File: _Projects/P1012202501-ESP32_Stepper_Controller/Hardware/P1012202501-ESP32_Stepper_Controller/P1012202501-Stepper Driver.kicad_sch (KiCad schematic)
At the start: 17 parts, among them CN6 KHS4B-PH-SM4-TB(LF)(SN), CN7 KPTBP04R1-500-04BE, IC6 UDRV8825PWPR

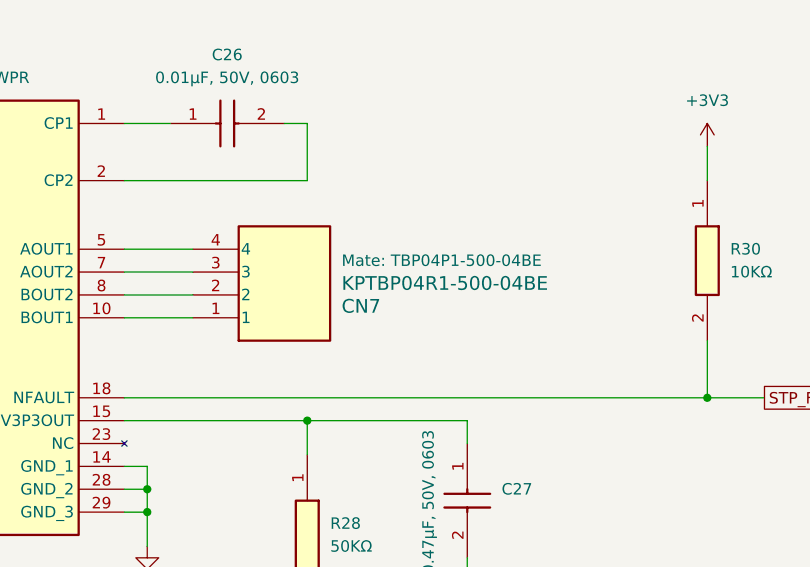
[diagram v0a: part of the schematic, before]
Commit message: Added new content and changes from stream.
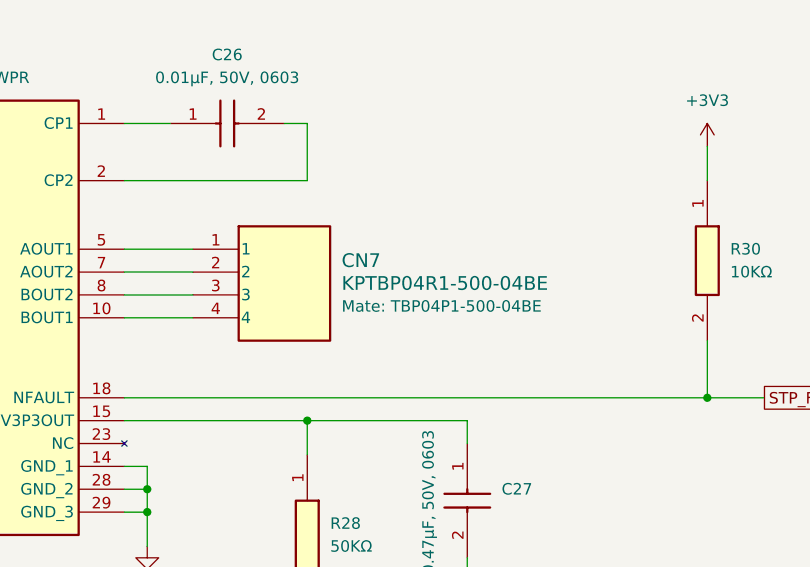
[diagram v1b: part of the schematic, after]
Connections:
- net at CN7.1: now also IC6.5 (AOUT1); no longer IC6.10 (BOUT1)
- net at CN7.2: now also IC6.7 (AOUT2); no longer IC6.8 (BOUT2)
- net at CN7.3: now also IC6.8 (BOUT2); no longer IC6.7 (AOUT2)
- net at CN7.4: now also IC6.10 (BOUT1); no longer IC6.5 (AOUT1)

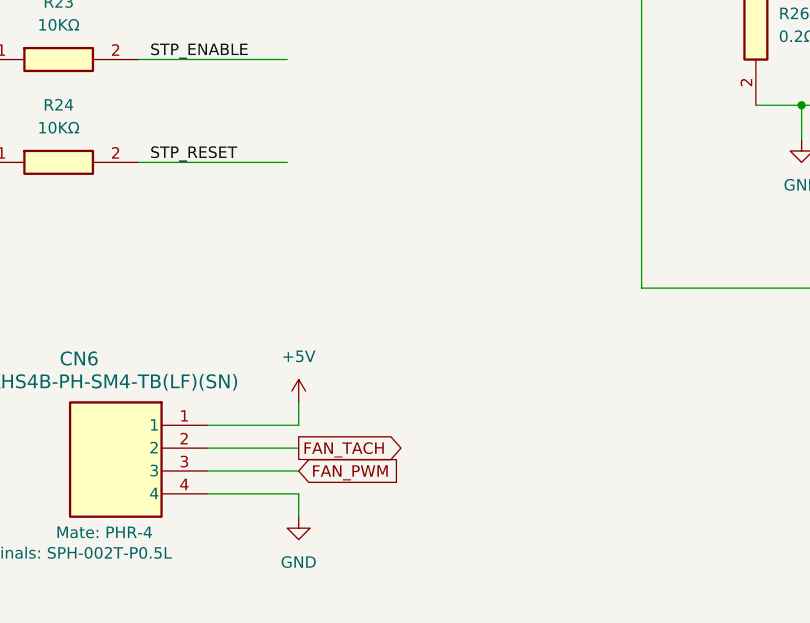
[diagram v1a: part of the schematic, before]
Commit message: Added items from latest stream.
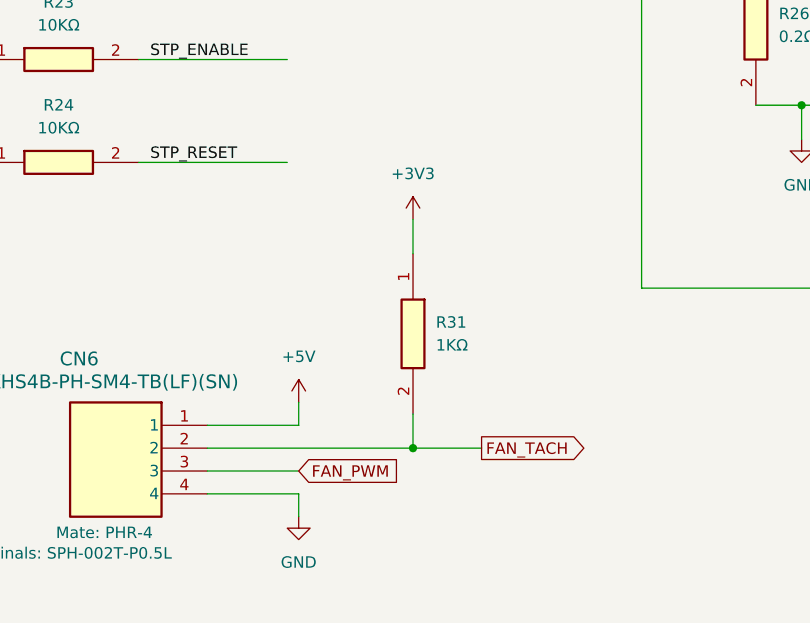
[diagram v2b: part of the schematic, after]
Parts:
- added R31: RC06031K0075AAA, COMPONENTS:RES-0603, symbol COMPONENTS:RC06031K0075AAA
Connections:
- net +3V3: now also R31.1
- net FAN_TACH: now also R31.2
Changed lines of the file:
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@@
 	)
 	(junction
+		(at 80.01 171.45)
+		(diameter 0)
+		(color 0 0 0 0)
+	)
+	(junction
 		(at 72.39 69.85)
 		(diameter 0)
@@
 	(wire
 		(pts
+			(xy 80.01 146.05) (xy 80.01 149.86)
+		)
+		(stroke
+			(width 0)
+			(type default)
+		)
+	)
+	(wire
+		(pts
 			(xy 170.18 113.03) (xy 172.72 113.03)
 		)
@@
 	(wire
 		(pts
+			(xy 80.01 171.45) (xy 87.63 171.45)
+		)
+		(stroke
+			(width 0)
+			(type default)
+		)
+	)
+	(wire
+		(pts
 			(xy 105.41 106.68) (xy 105.41 153.67)
 		)
@@
 	(wire
 		(pts
-			(xy 57.15 171.45) (xy 67.31 171.45)
+			(xy 57.15 171.45) (xy 80.01 171.45)
 		)
 		(stroke
@@
 	(wire
 		(pts
+			(xy 80.01 167.64) (xy 80.01 171.45)
+		)
+		(stroke
+			(width 0)
+			(type default)
+		)
+	)
+	(wire
+		(pts
 			(xy 234.95 72.39) (xy 234.95 76.2)
 		)
@@
 	(global_label "FAN_TACH"
 		(shape output)
-		(at 67.31 171.45 0)
+		(at 87.63 171.45 0)
 		(fields_autoplaced yes)
 		(effects
@@
 		)
 		(property "Intersheetrefs" "${INTERSHEET_REFS}"
-			(at 79.4272 171.45 0)
+			(at 99.7472 171.45 0)
 			(effects
 				(font
@@
 	)
 	(symbol
+		(lib_id "COMPONENTS:RC06031K0075AAA")
+		(at 80.01 149.86 270)
+		(unit 1)
+		(exclude_from_sim no)
+		(in_bom yes)
+		(on_board yes)
+		(dnp no)
+		(fields_autoplaced yes)
+		(property "Reference" "R31"
+			(at 82.55 157.4799 90)
+			(effects
+				(font
+					(size 1.27 1.27)
+				)
+				(justify left)
+			)
+		)
+		(property "Value" "RC06031K0075AAA"
+			(at 73.914 151.384 0)
+			(effects
+				(font
+					(size 1.27 1.27)
+				)
+				(justify left top)
+				(hide yes)
+			)
+		)
+		(property "Footprint" "COMPONENTS:RES-0603"
+			(at -16.18 163.83 0)
+			(effects
+				(font
+					(size 1.27 1.27)
+				)
+				(justify left top)
+				(hide yes)
+			)
+		)
+		(property "Datasheet" ""
+			(at -116.18 163.83 0)
+			(effects
+				(font
+					(size 1.27 1.27)
+				)
+				(justify left top)
+				(hide yes)
+			)
+		)
+		(property "Description" "Resistor, Chip, 0603, 1KΩ, 75V, 5%, -55°C to 155°C, RoHS, AEC-Q200"
+			(at 70.866 153.924 0)
+			(effects
+				(font
+					(size 1.27 1.27)
+				)
+				(hide yes)
+			)
+		)
+		(property "Manufacturer 1" "Yageo"
+			(at 64.516 147.32 0)
+			(effects
+				(font
+					(size 1.27 1.27)
+				)
+				(hide yes)
+			)
+		)
+		(property "Manufacturer 1 P/N" "SR0603JR-071KL"
+			(at 66.802 156.972 0)
+			(effects
+				(font
+					(size 1.27 1.27)
+				)
+				(hide yes)
+			)
+		)
+		(property "Vendor 1a" "Mouser"
+			(at 82.296 130.048 0)
+			(effects
+				(font
+					(size 1.27 1.27)
+				)
+				(hide yes)
+			)
+		)
+		(property "Vendor 1a P/N" "603-SR0603JR-071KL"
+			(at 90.424 146.05 0)
+			(effects
+				(font
+					(size 1.27 1.27)
+				)
+				(hide yes)
+			)
+		)
+		(property "Vendor 1a Cost LV" "0.11"
+			(at 79.756 131.064 0)
+			(effects
+				(font
+					(size 1.27 1.27)
+				)
+				(hide yes)
+			)
+		)
+		(property "Vendor 1a Cost HV" "0.031"
+			(at 86.36 131.572 0)
+			(effects
+				(font
+					(size 1.27 1.27)
+				)
+				(hide yes)
+			)
+		)
+		(property "Val" "1KΩ"
+			(at 82.55 160.0199 90)
+			(effects
+				(font
+					(size 1.27 1.27)
+				)
+				(justify left)
+			)
+		)
+		(pin "1"
+		)
+		(pin "2"
+		)
+		(instances
+			(project ""
+				(path "/27f0531a-0a2b-4c68-af50-4332bf165b5a/2932f4ee-8c5b-459c-9bd5-5a172fd29c3b"
+					(reference "R31")
+					(unit 1)
+				)
+			)
+		)
+	)
+	(symbol
 		(lib_id "COMPONENTS:CC0603104050AAAX7R")
 		(at 55.88 74.93 270)
@@
 					(unit 1)
 				)
+			)
+		)
+	)
+	(symbol
+		(lib_id "power:+3V3")
+		(at 80.01 146.05 0)
+		(unit 1)
+		(exclude_from_sim no)
+		(in_bom yes)
+		(on_board yes)
+		(dnp no)
+		(fields_autoplaced yes)
+		(property "Reference" "#PWR073"
+			(at 80.01 149.86 0)
+			(effects
+				(font
+					(size 1.27 1.27)
+				)
+				(hide yes)
+			)
+		)
+		(property "Value" "+3V3"
+			(at 80.01 140.97 0)
+			(effects
+				(font
+					(size 1.27 1.27)
+				)
+			)
+		)
+		(property "Footprint" ""
+			(at 80.01 146.05 0)
+			(effects
+				(font
+					(size 1.27 1.27)
+				)
+				(hide yes)
+			)
+		)
+		(property "Datasheet" ""
+			(at 80.01 146.05 0)
+			(effects
+				(font
+					(size 1.27 1.27)
+				)
+				(hide yes)
+			)
+		)
+		(property "Description" "Power symbol creates a global label with name \"+3V3\""
+			(at 80.01 146.05 0)
+			(effects
+				(font
+					(size 1.27 1.27)
+				)
+				(hide yes)
+			)
+		)
+		(pin "1"
+		)
+		(instances
+			(project "P1012202501-ESP32_Stepper_Controller"
+				(path "/27f0531a-0a2b-4c68-af50-4332bf165b5a/2932f4ee-8c5b-459c-9bd5-5a172fd29c3b"
+					(reference "#PWR073")
+					(unit 1)
+				)
